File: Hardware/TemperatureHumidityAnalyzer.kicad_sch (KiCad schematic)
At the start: 33 parts, among them J1 Power, J2 SSD1306 Display, J3 SWD, SW1 SW_Push, SW2 SW_Nidec_CAS-120A1, U1 AMS1117-3.3, U2 HDC2010YPAR, U3 STM32L432KCU6, Y1 8MHz Crystal

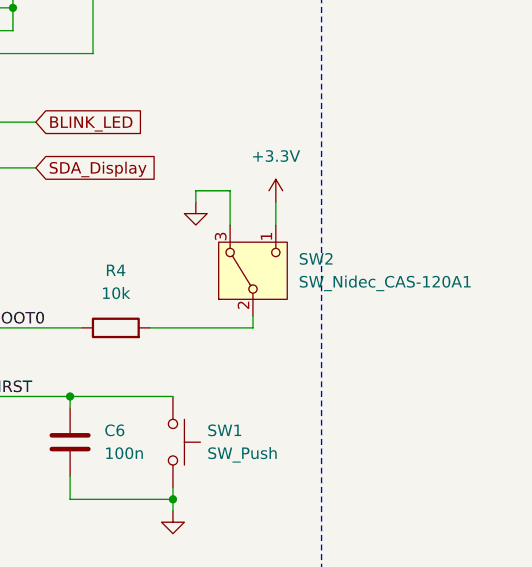
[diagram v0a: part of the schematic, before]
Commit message: Generate manufacturing files
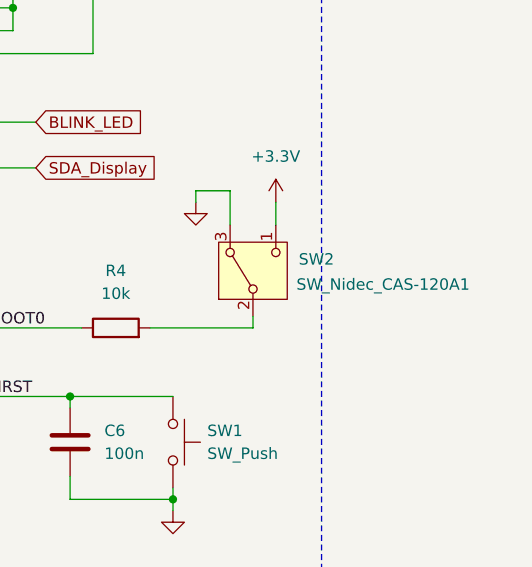
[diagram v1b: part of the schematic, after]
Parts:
- J2: Link (none) -> https://www.amazon.ca/0-96inch-Module-Display-SSD1306-Drive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
